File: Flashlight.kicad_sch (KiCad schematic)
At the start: 11 parts

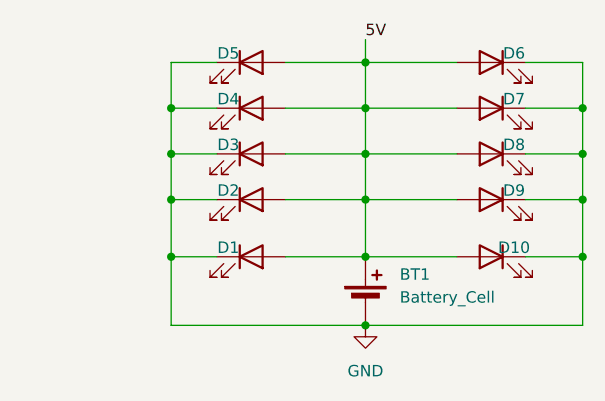
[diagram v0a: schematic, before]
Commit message: Finalized Kicad PCB Design
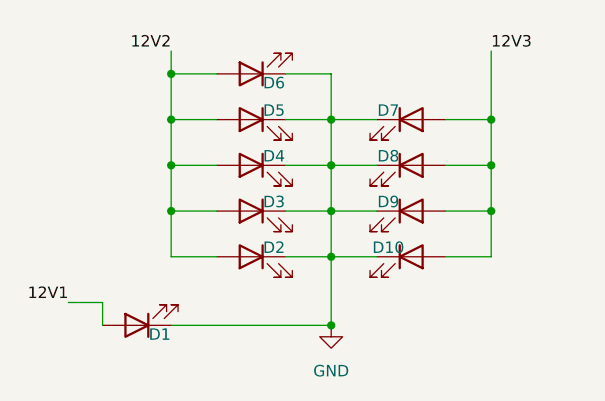
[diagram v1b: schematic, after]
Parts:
- removed BT1: Battery_Cell, symbol Device:Battery_Cell
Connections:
- net 5V renamed 12V2
- net 12V2: no longer D1.2 (A), D10.2 (A), D7.2 (A), D8.2 (A), D9.2 (A)
- new net 12V1: D1.2 (A)
- new net 12V3: D10.2 (A), D7.2 (A), D8.2 (A), D9.2 (A)
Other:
- moved on the sheet: D1, D10, D2, D3, D4, D5, D6, D7, D8, D9
